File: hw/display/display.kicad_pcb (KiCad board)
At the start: 4 copper layers, 37 x 29 mm, 22 parts, among them J1 Input, J2 Output, U1 SN65LVDS822, U2 SN74LVC00ARGY

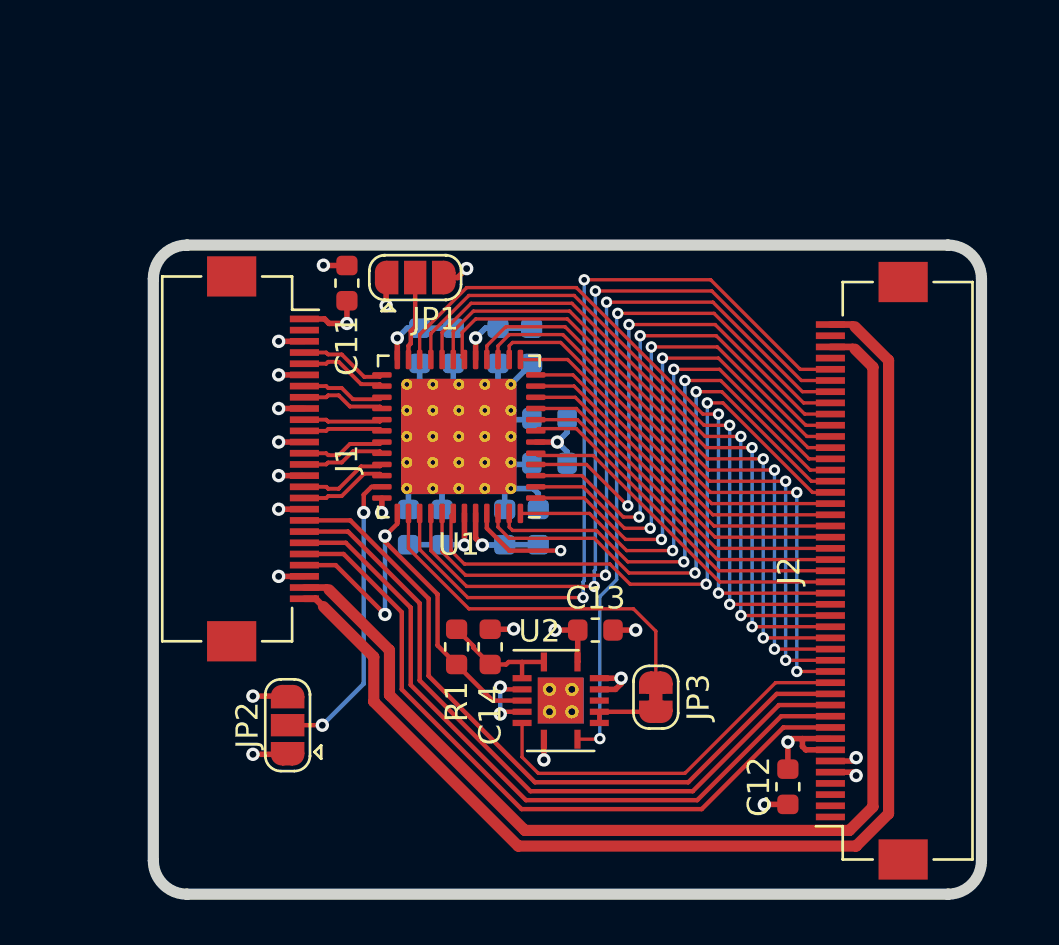
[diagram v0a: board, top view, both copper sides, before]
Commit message: temp commit for merge
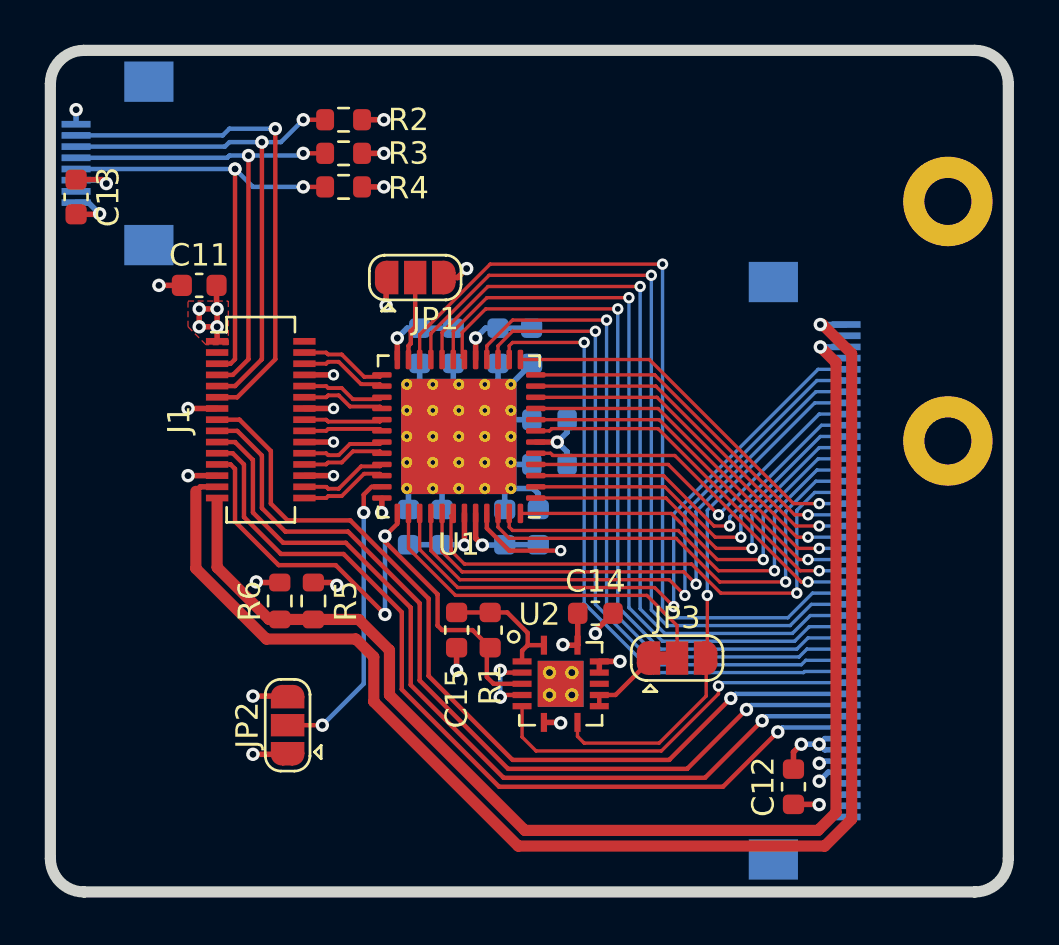
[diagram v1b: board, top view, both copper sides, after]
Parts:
- added C13: 0.1uF, Capacitor_SMD:C_0603_1608Metric, F.Cu at (106.5, 77.8)
- added J3: Touch, Connector_FFC-FPC:Hirose_FH12-8S-0.5SH_1x08-1MP_P0.50mm_Horizontal, B.Cu at (108.4, 76.3)
- added J4: Spacer, footprints:Spacer, F.Cu at (145.5, 78.0)
- added J5: Spacer, footprints:Spacer, F.Cu at (145.5, 88.8)
- added R2: DNP, Resistor_SMD:R_0603_1608Metric, F.Cu at (118.5, 74.4)
- added R3: DNP, Resistor_SMD:R_0603_1608Metric, F.Cu at (118.5, 75.9)
- added R4: DNP, Resistor_SMD:R_0603_1608Metric, F.Cu at (118.5, 77.4)
- added R5: DNP, Resistor_SMD:R_0603_1608Metric, F.Cu at (117.2, 95.9)
- added R6: DNP, Resistor_SMD:R_0603_1608Metric, F.Cu at (115.7, 95.9)
- J1: footprint Connector_FFC-FPC:Hirose_FH12-26S-0.5SH_1x26-1MP_P0.50mm_Horizontal -> Connector_Molex:Molex_SlimStack_55560-0301_2x15_P0.50mm_Vertical
- J2: value Output -> Display; moved to B.Cu
- JP3: footprint Jumper:SolderJumper-2_P1.3mm_Bridged_RoundedPad1.0x1.5mm -> Jumper:SolderJumper-3_P1.3mm_Bridged12_RoundedPad1.0x1.5mm
- U2: footprint Package_DFN_QFN:Texas_S-PVQFN-N14_ThermalVias -> footprints:Texas_S-PVQFN-N14_ThermalVias
- moved C11 6.60 mm to (112.0, 81.8), turned to 180 degrees
- moved J2 3.00 mm to (139.1, 94.5)
- moved JP3 1.99 mm to (133.4, 98.5), turned to 0 degrees
- moved J1 1.75 mm to (114.8, 87.8), turned to 90 degrees
- moved C15 1.68 mm to (123.5, 97.2), turned to 270 degrees
- moved R1 1.68 mm to (125.0, 97.2)
- moved C14 0.75 mm to (129.8, 96.5)
- moved U2 0.75 mm to (128.2, 99.6)
- moved C12 0.25 mm to (138.6, 104.2)
- renumbered C13 to C14, C14 to C15
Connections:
- J1 pad 10: /LVDS_A2N -> /LVDS_A1N
- J1 pad 11: /LVDS_A2P -> CTP.RST
- J1 pad 12: GND -> /LVDS_A1P
- J1 pad 13: /LVDS_CLKN -> GND
- J1 pad 14: /LVDS_CLKP -> GND
- J1 pad 15: GND -> SPI.CS
- J1 pad 16: /LVDS_A3N -> /LVDS_A2N
- J1 pad 17: /LVDS_A3P -> SPI.SCK
- J1 pad 18: GND -> /LVDS_A2P
- J1 pad 19: SPI.CS -> SPI.MOSI
- J1 pad 20: SPI.SCK -> GND
- J1 pad 21: SPI.MOSI -> SPI.MISO
- J1 pad 22: SPI.MISO -> /LVDS_CLKN
- J1 pad 24: GND -> /LVDS_CLKP
- J1 pad 25: LED_K -> GND
- J1 pad 26: LED_A -> GND
- J1 pad 3: GND -> Net-(J1-Pad3)
- J1 pad 5: /LVDS_A0P -> CTP.SCL
- J1 pad 6: GND -> /LVDS_A0P
- J1 pad 7: /LVDS_A1N -> CTP.SDA
- J1 pad 8: /LVDS_A1P -> GND
- J1 pad 9: GND -> CTP.INT
- JP3 pad 1: /DISP_EN_IC -> Net-(JP3-Pad1)
- JP3 pad 2: Net-(JP3-Pad2) -> /DISP_DE_INV
- U1 pad 38: /DISP_EN_IC -> /DISP_DE_INV
- U2 pad 10: Net-(JP3-Pad2) -> Net-(JP3-Pad1)
- U2 pad 9: Net-(JP3-Pad2) -> Net-(JP3-Pad1)
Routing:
- net CTP.INT: track 0.00 -> 23.8 mm, vias 0 -> 2
- net CTP.RST: track 0.00 -> 22.6 mm, vias 0 -> 1
- net CTP.SDA: track 0.00 -> 22.0 mm, vias 0 -> 2
- net CTP.SCL: track 0.00 -> 20.8 mm, vias 0 -> 2
- net /DISP_EN_IC: track 16.4 -> 0.00 mm
- net /DISP_DE_INV: track 0.00 -> 16.4 mm
- net LED_A: track 56.0 -> 64.5 mm, vias 0 -> 1
- net /DISP_VSYNC: track 36.7 -> 28.5 mm, vias 2 -> 1
- net /DISP_HSYNC: track 35.0 -> 27.2 mm, vias 2 -> 1
- net /DISP_DE: track 31.5 -> 23.9 mm, vias 2 -> 1
- net /DISP_PCLK: track 33.3 -> 25.8 mm, vias 2 -> 1
- net ENABLE: track 19.9 -> 27.2 mm
- net +3V3: track 31.6 -> 38.8 mm, vias 10 -> 18
- net SPI.MOSI: track 31.8 -> 38.8 mm, vias 0 -> 1
- net SPI.MISO: track 31.8 -> 38.8 mm, vias 0 -> 1
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- added copper zone on F.Cu, net +3V3
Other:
- board size 37 x 29 mm -> 42.8 x 37.6 mm
